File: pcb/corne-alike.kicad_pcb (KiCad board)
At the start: 2 copper layers, 130.3 x 85.3 mm, 47 parts, among them J1 Conn_01x02_Socket, SW1 SW_PUSH, SW10 SW_PUSH, SW11 SW_PUSH, SW12 SW_PUSH, SW13 SW_PUSH, SW14 SW_PUSH, SW15 SW_PUSH, SW16 SW_PUSH, SW17 SW_PUSH, SW18 SW_PUSH, SW19 SW_PUSH, SW2 SW_PUSH, SW20 SW_PUSH, SW21 SW_PUSH, SW3 SW_PUSH, SW4 SW_PUSH, SW5 SW_PUSH, SW6 SW_PUSH, SW7 SW_PUSH, SW8 SW_PUSH, SW9 SW_PUSH, U1 ProMicro

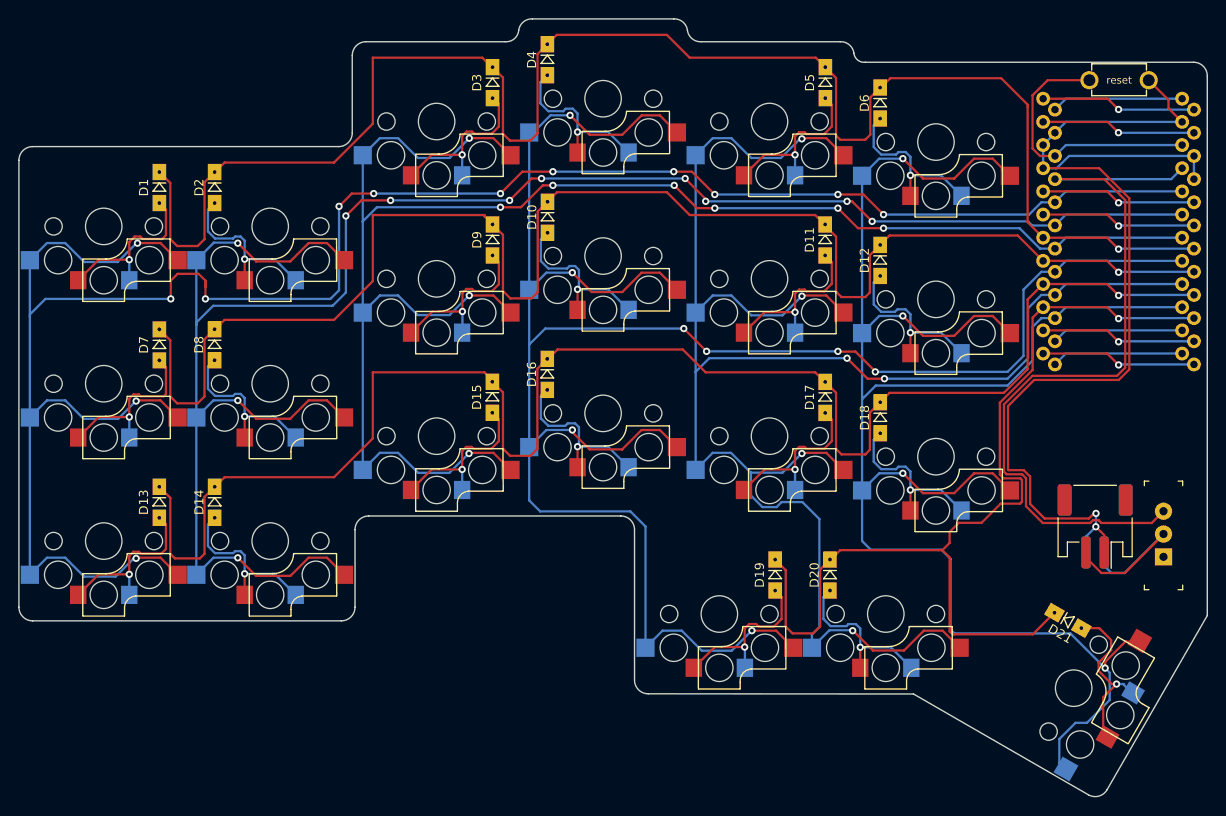
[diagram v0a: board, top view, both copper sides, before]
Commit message: Clean up tracks
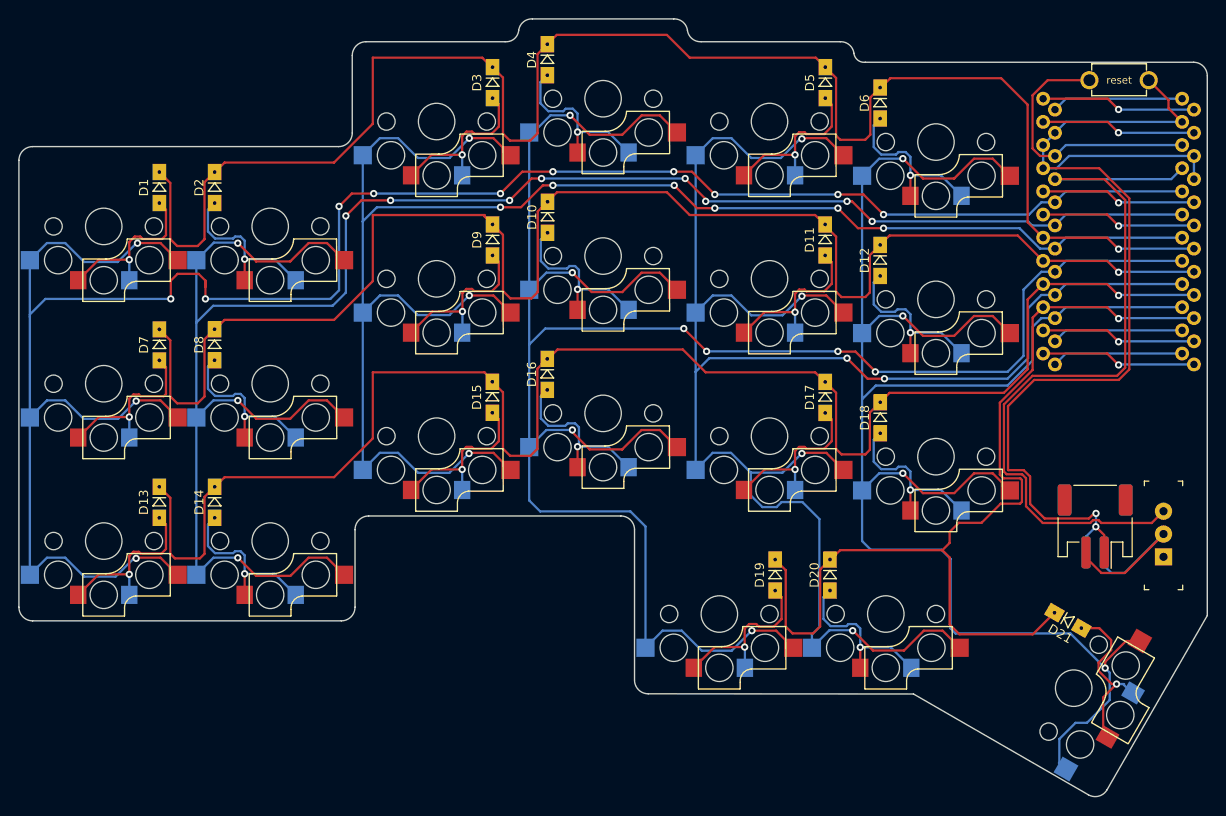
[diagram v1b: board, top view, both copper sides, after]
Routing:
- net Net-(#FLG01-pwr): track 21.3 -> 19.3 mm
- net col5: track 197.1 -> 198.6 mm
- net row3: track 108.7 -> 108.1 mm
